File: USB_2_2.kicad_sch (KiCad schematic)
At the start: 14 parts, among them J3 USB_C_Receptacle_USB2.0, U15 USB3300-EZK, X1 ECS-2520MV-xxx-xx

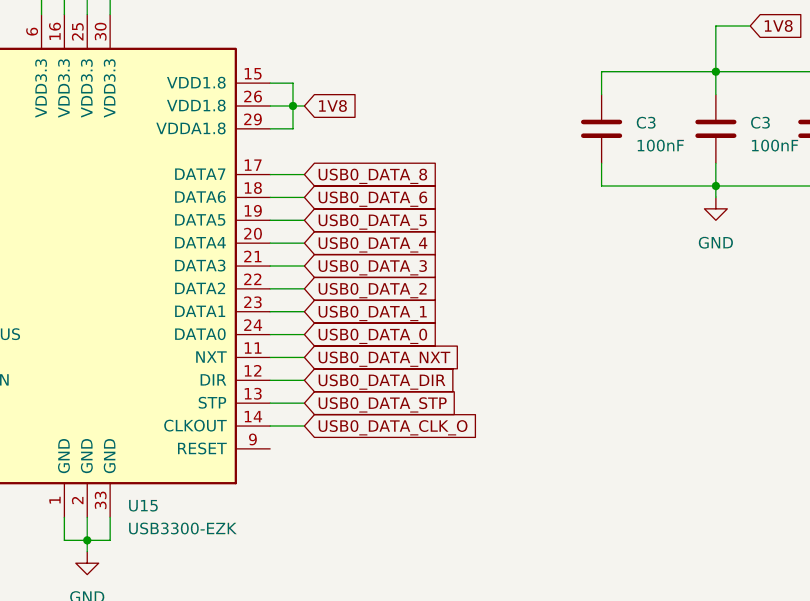
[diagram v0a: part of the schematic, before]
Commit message: usb and stuff
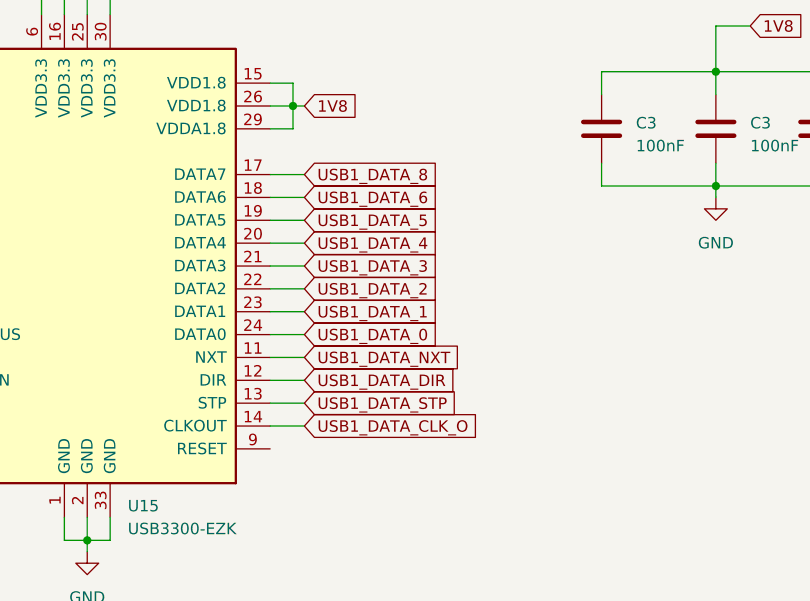
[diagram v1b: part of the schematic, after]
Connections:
- net USB0_DATA_0 renamed USB1_DATA_0
- net USB0_DATA_1 renamed USB1_DATA_1
- net USB0_DATA_2 renamed USB1_DATA_2
- net USB0_DATA_3 renamed USB1_DATA_3
- net USB0_DATA_4 renamed USB1_DATA_4
- net USB0_DATA_5 renamed USB1_DATA_5
- net USB0_DATA_6 renamed USB1_DATA_6
- net USB0_DATA_8 renamed USB1_DATA_8
- net USB0_DATA_CLK_O renamed USB1_DATA_CLK_O
- net USB0_DATA_DIR renamed USB1_DATA_DIR
- net USB0_DATA_NXT renamed USB1_DATA_NXT
- net USB0_DATA_STP renamed USB1_DATA_STP
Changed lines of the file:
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@@
     (effects (font (size 1.27 1.27)) (justify left bottom))
   )
-  (global_label "USB0_DATA_STP" (shape input) (at 194.31 100.33 0) (fields_autoplaced)
+  (global_label "USB1_DATA_STP" (shape input) (at 194.31 100.33 0) (fields_autoplaced)
     (effects (font (size 1.27 1.27)) (justify left))
     (property "Intersheetrefs" "${INTERSHEET_REFS}" (at 212.0324 100.33 0)
@@
     )
   )
-  (global_label "USB0_DATA_5" (shape input) (at 194.31 80.01 0) (fields_autoplaced)
+  (global_label "USB1_DATA_5" (shape input) (at 194.31 80.01 0) (fields_autoplaced)
     (effects (font (size 1.27 1.27)) (justify left))
     (property "Intersheetrefs" "${INTERSHEET_REFS}" (at 209.7948 80.01 0)
@@
     )
   )
-  (global_label "USB0_DATA_1" (shape input) (at 194.31 90.17 0) (fields_autoplaced)
+  (global_label "USB1_DATA_1" (shape input) (at 194.31 90.17 0) (fields_autoplaced)
     (effects (font (size 1.27 1.27)) (justify left))
     (property "Intersheetrefs" "${INTERSHEET_REFS}" (at 209.7948 90.17 0)
@@
     )
   )
-  (global_label "USB0_DATA_2" (shape input) (at 194.31 87.63 0) (fields_autoplaced)
+  (global_label "USB1_DATA_2" (shape input) (at 194.31 87.63 0) (fields_autoplaced)
     (effects (font (size 1.27 1.27)) (justify left))
     (property "Intersheetrefs" "${INTERSHEET_REFS}" (at 209.7948 87.63 0)
@@
     )
   )
-  (global_label "USB0_DATA_NXT" (shape input) (at 194.31 95.25 0) (fields_autoplaced)
+  (global_label "USB1_DATA_NXT" (shape input) (at 194.31 95.25 0) (fields_autoplaced)
     (effects (font (size 1.27 1.27)) (justify left))
     (property "Intersheetrefs" "${INTERSHEET_REFS}" (at 212.0929 95.25 0)
@@
     )
   )
-  (global_label "USB0_DATA_8" (shape input) (at 194.31 74.93 0) (fields_autoplaced)
+  (global_label "USB1_DATA_8" (shape input) (at 194.31 74.93 0) (fields_autoplaced)
     (effects (font (size 1.27 1.27)) (justify left))
     (property "Intersheetrefs" "${INTERSHEET_REFS}" (at 209.7948 74.93 0)
@@
     )
   )
-  (global_label "USB0_DATA_4" (shape input) (at 194.31 82.55 0) (fields_autoplaced)
+  (global_label "USB1_DATA_4" (shape input) (at 194.31 82.55 0) (fields_autoplaced)
     (effects (font (size 1.27 1.27)) (justify left))
     (property "Intersheetrefs" "${INTERSHEET_REFS}" (at 209.7948 82.55 0)
@@
     )
   )
-  (global_label "USB0_DATA_CLK_O" (shape input) (at 194.31 102.87 0) (fields_autoplaced)
+  (global_label "USB1_DATA_CLK_O" (shape input) (at 194.31 102.87 0) (fields_autoplaced)
     (effects (font (size 1.27 1.27)) (justify left))
     (property "Intersheetrefs" "${INTERSHEET_REFS}" (at 214.4515 102.87 0)
@@
     )
   )
-  (global_label "USB0_DATA_6" (shape input) (at 194.31 77.47 0) (fields_autoplaced)
+  (global_label "USB1_DATA_6" (shape input) (at 194.31 77.47 0) (fields_autoplaced)
     (effects (font (size 1.27 1.27)) (justify left))
     (property "Intersheetrefs" "${INTERSHEET_REFS}" (at 209.7948 77.47 0)
@@
     )
   )
-  (global_label "USB0_DATA_3" (shape input) (at 194.31 85.09 0) (fields_autoplaced)
+  (global_label "USB1_DATA_3" (shape input) (at 194.31 85.09 0) (fields_autoplaced)
     (effects (font (size 1.27 1.27)) (justify left))
     (property "Intersheetrefs" "${INTERSHEET_REFS}" (at 209.7948 85.09 0)
@@
     )
   )
-  (global_label "USB0_DATA_0" (shape input) (at 194.31 92.71 0) (fields_autoplaced)
+  (global_label "USB1_DATA_0" (shape input) (at 194.31 92.71 0) (fields_autoplaced)
     (effects (font (size 1.27 1.27)) (justify left))
     (property "Intersheetrefs" "${INTERSHEET_REFS}" (at 209.7948 92.71 0)
@@
     )
   )
-  (global_label "USB0_DATA_DIR" (shape input) (at 194.31 97.79 0) (fields_autoplaced)
+  (global_label "USB1_DATA_DIR" (shape input) (at 194.31 97.79 0) (fields_autoplaced)
     (effects (font (size 1.27 1.27)) (justify left))
     (property "Intersheetrefs" "${INTERSHEET_REFS}" (at 211.7301 97.79 0)
